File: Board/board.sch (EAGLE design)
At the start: 49 parts, among them IC1 L297, IC2 MEGA32-P, IC3 L298, J1 +12V, Q1 BC639, Q3 BC639, U1 MCP9808MSOP, X1 WATER_PUMP, X2 FAN, X5 SM_CD, X6 SM_AB

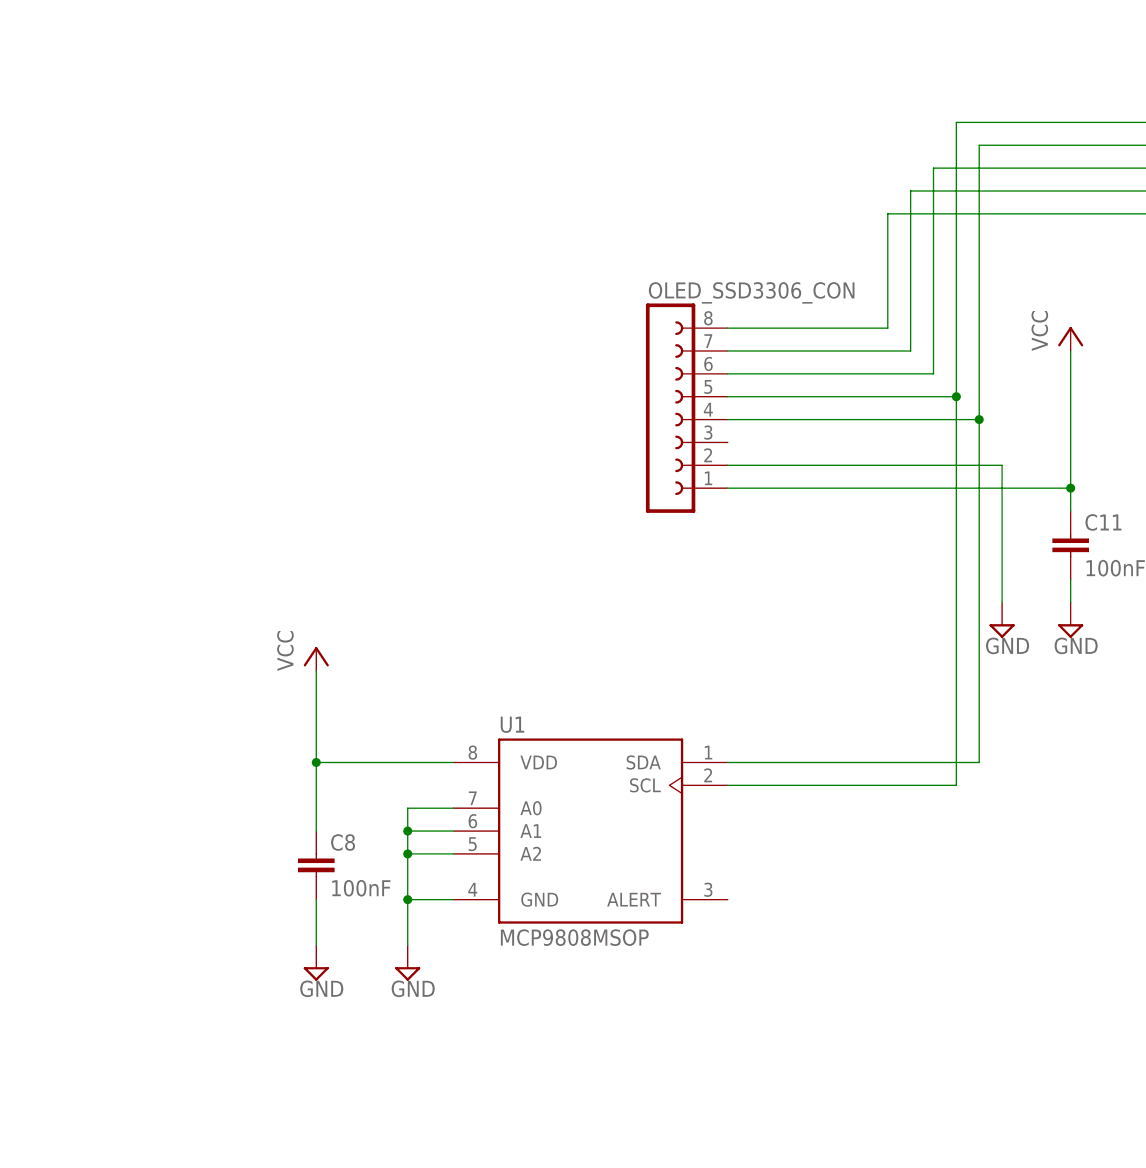
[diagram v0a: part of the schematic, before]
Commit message: ds
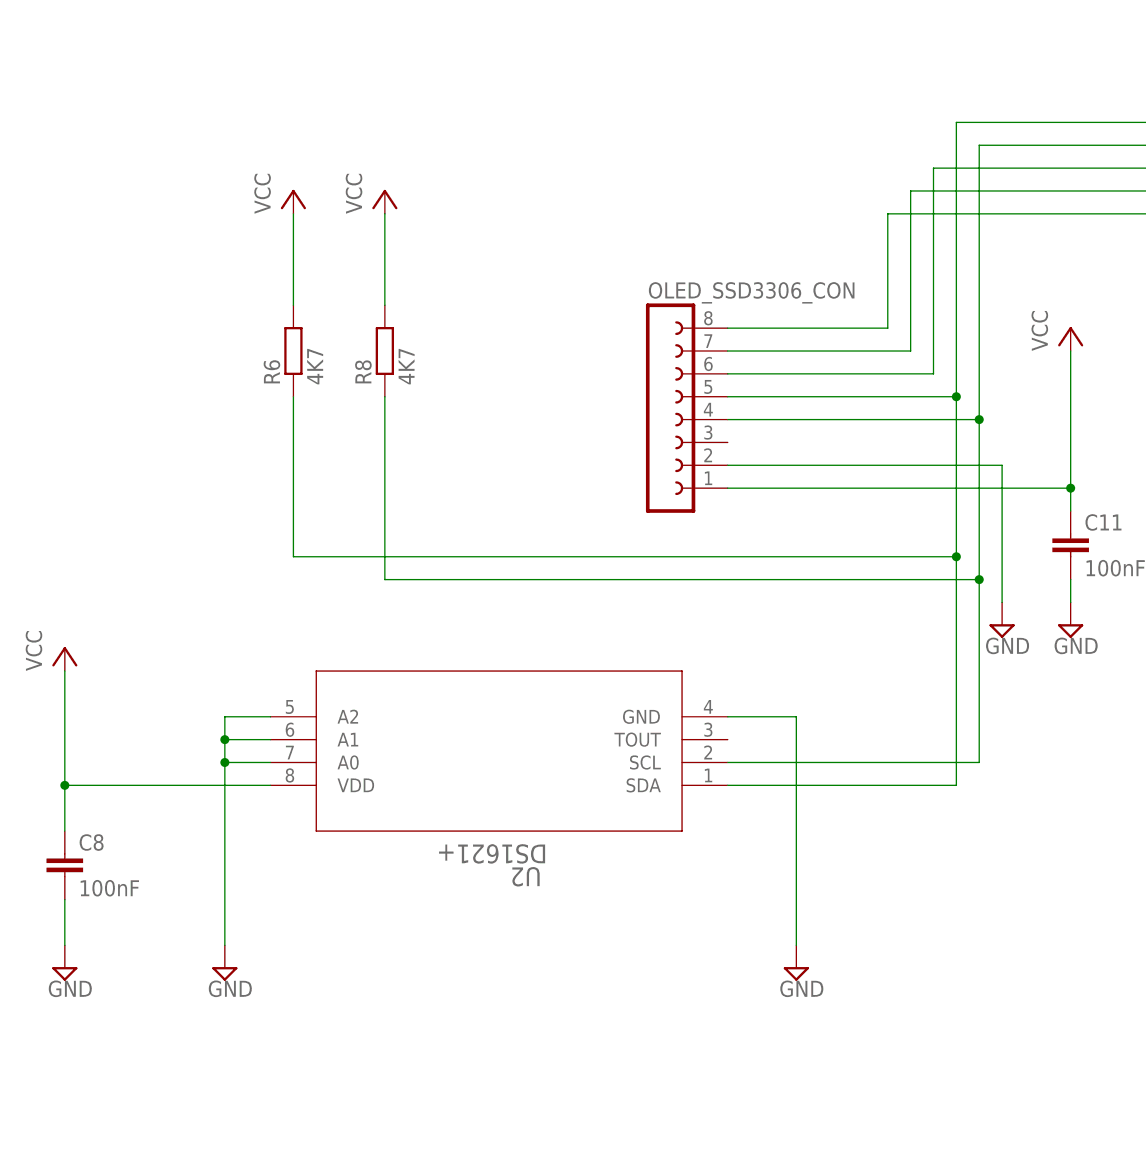
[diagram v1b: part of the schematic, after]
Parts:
- removed U1: MCP9808MSOP, MCP9808:MCP9808MSOP
- added R6, R8: 4K7, rcl:R-EU_0207/12
- added U2: DS1621+, ds1621p:DS1621+
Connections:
- net GND: now also U2.A0, U2.A1, U2.A2, U2.GND; no longer U1.A0, U1.A1, U1.A2, U1.GND
- net N$35: now also R8.1, U2.SCL; no longer U1.SDA
- net N$36: now also R6.1, U2.SDA; no longer U1.SCL
- net VCC: now also R6.2, R8.2, U2.VDD; no longer U1.VDD
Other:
- moved on the sheet: C8
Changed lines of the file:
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@@
 <setting verticaltext="up"/>
 </settings>
-<grid distance="0.1" unitdist="inch" unit="inch" style="dots" multiple="1" display="yes" altdistance="0.01" altunitdist="inch" altunit="inch"/>
+<grid distance="0.1" unitdist="inch" unit="inch" style="lines" multiple="1" display="no" altdistance="0.01" altunitdist="inch" altunit="inch"/>
 <layers>
 <layer number="1" name="Top" color="4" fill="1" visible="no" active="no"/>
@@
 <part name="R12" library="rcl" deviceset="R-EU_" device="0207/12" value="330R"/>
 <part name="SUPPLY25" library="supply2" deviceset="GND" device=""/>
-<part name="U1" library="MCP9808" deviceset="MCP9808" device="MSOP"/>
 <part name="SUPPLY26" library="supply2" deviceset="GND" device=""/>
 <part name="C8" library="rcl" deviceset="C-EU" device="025-025X050" value="100nF"/>
@@
 <part name="CTRL_LED" library="led" deviceset="LED" device="5MM"/>
 <part name="VSS_LED" library="led" deviceset="LED" device="5MM"/>
+<part name="U2" library="ds1621p" deviceset="DS1621+" device=""/>
+<part name="SUPPLY31" library="supply2" deviceset="GND" device=""/>
+<part name="R6" library="rcl" deviceset="R-EU_" device="0207/12" value="4K7"/>
+<part name="R8" library="rcl" deviceset="R-EU_" device="0207/12" value="4K7"/>
+<part name="P+8" library="supply1" deviceset="VCC" device=""/>
+<part name="P+9" library="supply1" deviceset="VCC" device=""/>
 </parts>
 <sheets>
@@
 <instance part="R12" gate="G$1" x="12.7" y="-10.16" rot="R90"/>
 <instance part="SUPPLY25" gate="GND" x="12.7" y="-43.18"/>
-<instance part="U1" gate="G$1" x="-127" y="-132.08"/>
-<instance part="SUPPLY26" gate="GND" x="-147.32" y="-147.32"/>
-<instance part="C8" gate="G$1" x="-157.48" y="-134.62"/>
-<instance part="SUPPLY27" gate="GND" x="-157.48" y="-147.32"/>
-<instance part="P+14" gate="VCC" x="-157.48" y="-111.76"/>
+<instance part="SUPPLY26" gate="GND" x="-167.64" y="-147.32"/>
+<instance part="C8" gate="G$1" x="-185.42" y="-134.62"/>
+<instance part="SUPPLY27" gate="GND" x="-185.42" y="-147.32"/>
+<instance part="P+14" gate="VCC" x="-185.42" y="-111.76"/>
 <instance part="IC3" gate="L298" x="236.22" y="-167.64"/>
 <instance part="SUPPLY17" gate="GND" x="215.9" y="-198.12"/>
@@
 <instance part="CTRL_LED" gate="G$1" x="12.7" y="-27.94"/>
 <instance part="VSS_LED" gate="G$1" x="-45.72" y="116.84"/>
+<instance part="U2" gate="A" x="-109.22" y="-127" rot="R180"/>
+<instance part="SUPPLY31" gate="GND" x="-104.14" y="-147.32"/>
+<instance part="R6" gate="G$1" x="-160.02" y="-78.74" rot="R90"/>
+<instance part="R8" gate="G$1" x="-149.86" y="-78.74" rot="R90"/>
+<instance part="P+8" gate="VCC" x="-160.02" y="-60.96"/>
+<instance part="P+9" gate="VCC" x="-149.86" y="-60.96"/>
 </instances>
 <busses>
@@
 </segment>
 <segment>
-<pinref part="U1" gate="G$1" pin="GND"/>
-<wire x1="-142.24" y1="-139.7" x2="-147.32" y2="-139.7" width="0.1524" layer="91"/>
 <pinref part="SUPPLY26" gate="GND" pin="GND"/>
-<wire x1="-147.32" y1="-139.7" x2="-147.32" y2="-144.78" width="0.1524" layer="91"/>
-<pinref part="U1" gate="G$1" pin="A2"/>
-<wire x1="-142.24" y1="-134.62" x2="-147.32" y2="-134.62" width="0.1524" layer="91"/>
-<wire x1="-147.32" y1="-134.62" x2="-147.32" y2="-139.7" width="0.1524" layer="91"/>
-<junction x="-147.32" y="-139.7"/>
-<pinref part="U1" gate="G$1" pin="A1"/>
-<wire x1="-142.24" y1="-132.08" x2="-147.32" y2="-132.08" width="0.1524" layer="91"/>
-<wire x1="-147.32" y1="-132.08" x2="-147.32" y2="-134.62" width="0.1524" layer="91"/>
-<junction x="-147.32" y="-134.62"/>
-<pinref part="U1" gate="G$1" pin="A0"/>
-<wire x1="-142.24" y1="-129.54" x2="-147.32" y2="-129.54" width="0.1524" layer="91"/>
-<wire x1="-147.32" y1="-129.54" x2="-147.32" y2="-132.08" width="0.1524" layer="91"/>
-<junction x="-147.32" y="-132.08"/>
+<wire x1="-167.64" y1="-119.38" x2="-167.64" y2="-121.92" width="0.1524" layer="91"/>
+<pinref part="U2" gate="A" pin="A2"/>
+<wire x1="-167.64" y1="-121.92" x2="-167.64" y2="-124.46" width="0.1524" layer="91"/>
+<wire x1="-167.64" y1="-124.46" x2="-167.64" y2="-144.78" width="0.1524" layer="91"/>
+<wire x1="-167.64" y1="-119.38" x2="-162.56" y2="-119.38" width="0.1524" layer="91"/>
+<pinref part="U2" gate="A" pin="A1"/>
+<wire x1="-167.64" y1="-121.92" x2="-162.56" y2="-121.92" width="0.1524" layer="91"/>
+<junction x="-167.64" y="-121.92"/>
+<pinref part="U2" gate="A" pin="A0"/>
+<wire x1="-167.64" y1="-124.46" x2="-162.56" y2="-124.46" width="0.1524" layer="91"/>
+<junction x="-167.64" y="-124.46"/>
 </segment>
 <segment>
 <pinref part="C8" gate="G$1" pin="2"/>
 <pinref part="SUPPLY27" gate="GND" pin="GND"/>
-<wire x1="-157.48" y1="-139.7" x2="-157.48" y2="-144.78" width="0.1524" layer="91"/>
+<wire x1="-185.42" y1="-139.7" x2="-185.42" y2="-144.78" width="0.1524" layer="91"/>
 </segment>
 <segment>
@@
 <pinref part="SUPPLY30" gate="GND" pin="GND"/>
 <wire x1="-45.72" y1="111.76" x2="-45.72" y2="106.68" width="0.1524" layer="91"/>
+</segment>
+<segment>
+<pinref part="U2" gate="A" pin="GND"/>
+<wire x1="-111.76" y1="-119.38" x2="-104.14" y2="-119.38" width="0.1524" layer="91"/>
+<pinref part="SUPPLY31" gate="GND" pin="GND"/>
+<wire x1="-104.14" y1="-119.38" x2="-104.14" y2="-144.78" width="0.1524" layer="91"/>
 </segment>
 </net>
@@
 </segment>
 <segment>
-<pinref part="U1" gate="G$1" pin="VDD"/>
-<wire x1="-142.24" y1="-124.46" x2="-157.48" y2="-124.46" width="0.1524" layer="91"/>
 <pinref part="C8" gate="G$1" pin="1"/>
-<wire x1="-157.48" y1="-124.46" x2="-157.48" y2="-132.08" width="0.1524" layer="91"/>
 <pinref part="P+14" gate="VCC" pin="VCC"/>
-<wire x1="-157.48" y1="-114.3" x2="-157.48" y2="-124.46" width="0.1524" layer="91"/>
-<junction x="-157.48" y="-124.46"/>
+<wire x1="-185.42" y1="-114.3" x2="-185.42" y2="-127" width="0.1524" layer="91"/>
+<pinref part="U2" gate="A" pin="VDD"/>
+<wire x1="-185.42" y1="-127" x2="-185.42" y2="-132.08" width="0.1524" layer="91"/>
+<wire x1="-162.56" y1="-127" x2="-185.42" y2="-127" width="0.1524" layer="91"/>
+<junction x="-185.42" y="-127"/>
 </segment>
 <segment>
@@
 <wire x1="-73.66" y1="-93.98" x2="-73.66" y2="-96.52" width="0.1524" layer="91"/>
 <junction x="-73.66" y="-93.98"/>
+</segment>
+<segment>
+<pinref part="P+8" gate="VCC" pin="VCC"/>
+<pinref part="R6" gate="G$1" pin="2"/>
+<wire x1="-160.02" y1="-63.5" x2="-160.02" y2="-73.66" width="0.1524" layer="91"/>
+</segment>
+<segment>
+<pinref part="P+9" gate="VCC" pin="VCC"/>
+<pinref part="R8" gate="G$1" pin="2"/>
+<wire x1="-149.86" y1="-63.5" x2="-149.86" y2="-73.66" width="0.1524" layer="91"/>
 </segment>
 </net>
@@
 <wire x1="-83.82" y1="-86.36" x2="-111.76" y2="-86.36" width="0.1524" layer="91"/>
 <wire x1="-83.82" y1="-55.88" x2="-83.82" y2="-86.36" width="0.1524" layer="91"/>
-<pinref part="U1" gate="G$1" pin="SDA"/>
-<wire x1="-83.82" y1="-86.36" x2="-83.82" y2="-124.46" width="0.1524" layer="91"/>
+<wire x1="-83.82" y1="-86.36" x2="-83.82" y2="-104.14" width="0.1524" layer="91"/>
+<junction x="-83.82" y="-86.36"/>
+<pinref part="U2" gate="A" pin="SCL"/>
+<wire x1="-83.82" y1="-104.14" x2="-83.82" y2="-124.46" width="0.1524" layer="91"/>
 <wire x1="-83.82" y1="-124.46" x2="-111.76" y2="-124.46" width="0.1524" layer="91"/>
-<junction x="-83.82" y="-86.36"/>
+<pinref part="R8" gate="G$1" pin="1"/>
+<wire x1="-83.82" y1="-104.14" x2="-149.86" y2="-104.14" width="0.1524" layer="91"/>
+<wire x1="-149.86" y1="-104.14" x2="-149.86" y2="-83.82" width="0.1524" layer="91"/>
+<junction x="-83.82" y="-104.14"/>
 </segment>
 </net>
@@
 <wire x1="-86.36" y1="-53.34" x2="-86.36" y2="-83.82" width="0.1524" layer="91"/>
 <wire x1="-86.36" y1="-83.82" x2="-111.76" y2="-83.82" width="0.1524" layer="91"/>
-<wire x1="-86.36" y1="-83.82" x2="-86.36" y2="-127" width="0.1524" layer="91"/>
+<wire x1="-86.36" y1="-83.82" x2="-86.36" y2="-101.6" width="0.1524" layer="91"/>
 <junction x="-86.36" y="-83.82"/>
-<pinref part="U1" gate="G$1" pin="SCL"/>
+<pinref part="U2" gate="A" pin="SDA"/>
+<wire x1="-86.36" y1="-101.6" x2="-86.36" y2="-127" width="0.1524" layer="91"/>
 <wire x1="-86.36" y1="-127" x2="-111.76" y2="-127" width="0.1524" layer="91"/>
-</segment>
-</net>
+<pinref part="R6" gate="G$1" pin="1"/>
+<wire x1="-86.36" y1="-101.6" x2="-160.02" y2="-101.6" width="0.1524" layer="91"/>
+<wire x1="-160.02" y1="-101.6" x2="-160.02" y2="-83.82" width="0.1524" layer="91"/>
+<junction x="-86.36" y="-101.6"/>
+</segment>
+</net>
